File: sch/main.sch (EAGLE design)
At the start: 7 parts, among them U1 LTC3789EGNPBF

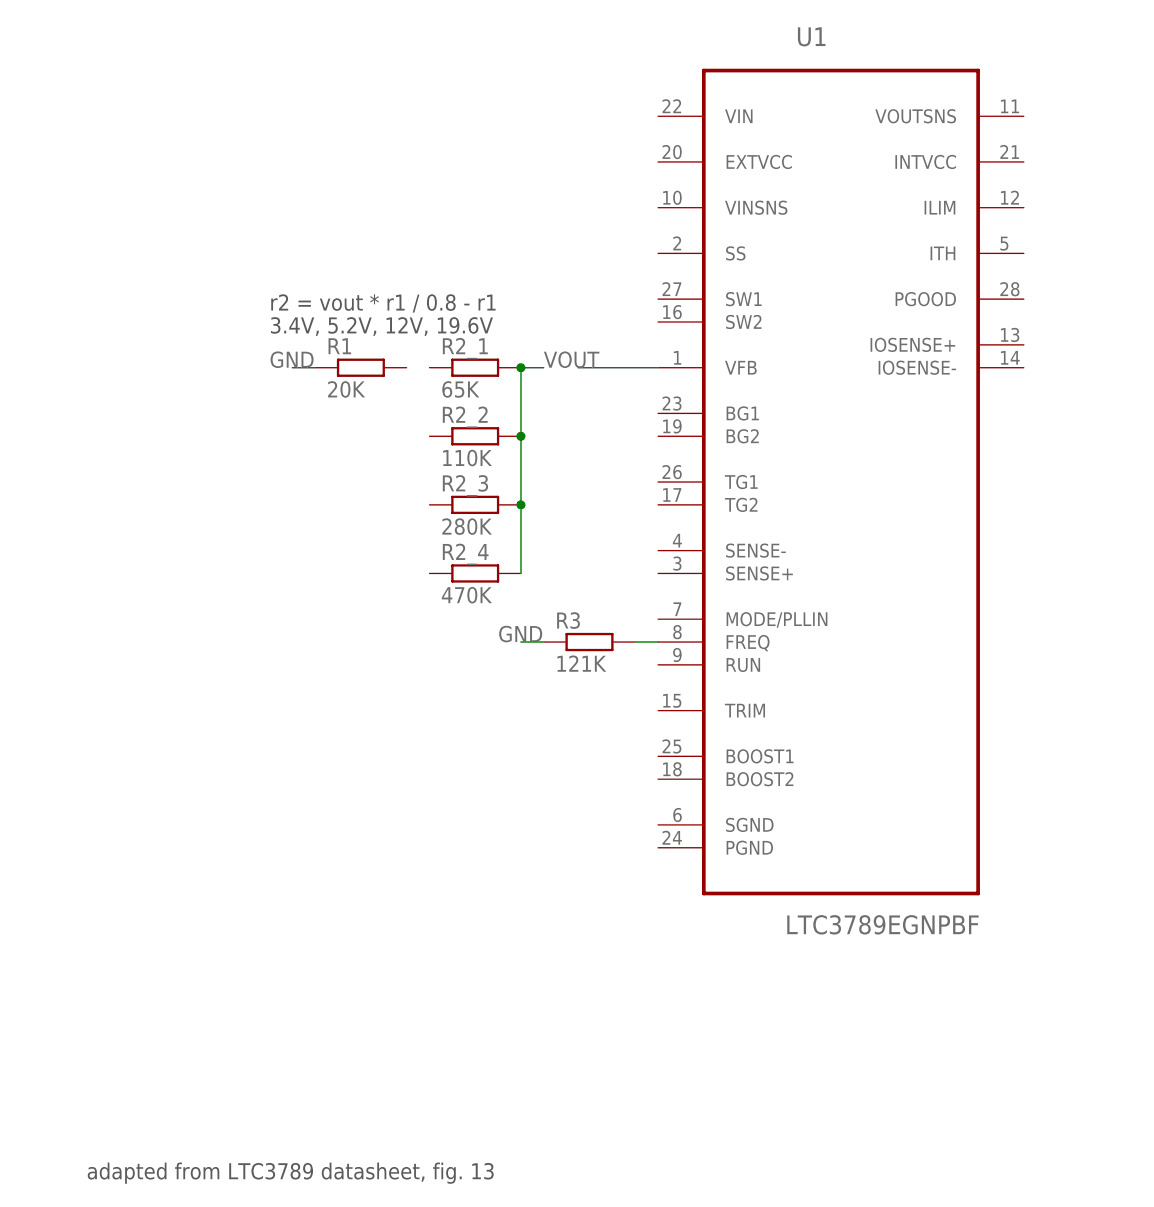
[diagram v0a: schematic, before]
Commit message: [ update ] sch
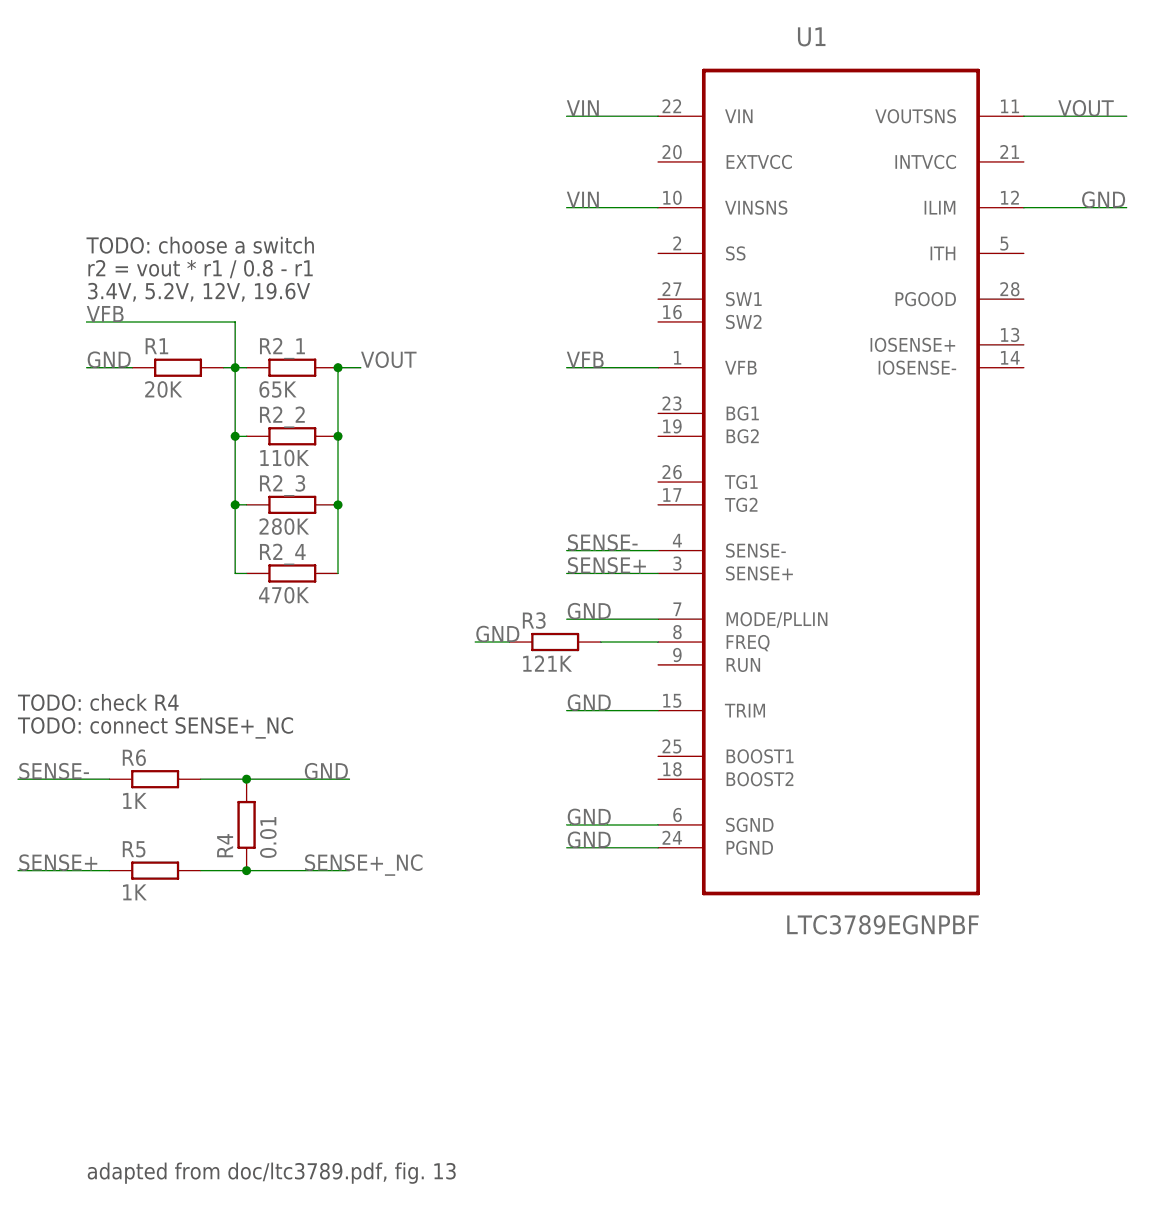
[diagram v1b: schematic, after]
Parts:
- added R4: 0.01, resistor:R-EU_R1206
- added R5, R6: 1K, resistor:R-EU_R1206
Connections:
- removed net N$3: U1.VFB
- new net SENSE+: R5.1, U1.SENSE+
- new net SENSE+_NC: R4.1, R5.2
- new net SENSE-: R6.1, U1.SENSE-
- new net VFB: R1.2, R2_1.1, R2_2.1, R2_3.1, R2_4.1, U1.VFB
- new net VIN: U1.VIN, U1.VINSNS
- net GND: now also R4.2, R6.2, U1.ILIM, U1.MODE/PLLIN, U1.PGND, U1.SGND, U1.TRIM
- net VOUT: now also U1.VOUTSNS
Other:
- note added: "TODO: check R4"
- note added: "TODO: choose a switch"
- note added: "TODO: connect SENSE+_NC"
- note added: "adapted from doc/ltc3789.pdf, fig. 13"
- note removed: "adapted from LTC3789 datasheet, fig. 13"
- moved on the sheet: R1, R2_1, R2_2, R2_3, R2_4, R3
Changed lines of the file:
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@@
 <part name="R2_3" library="resistor" deviceset="R-EU_" device="R1206" value="280K"/>
 <part name="R2_4" library="resistor" deviceset="R-EU_" device="R1206" value="470K"/>
+<part name="R4" library="resistor" deviceset="R-EU_" device="R1206" value="0.01"/>
+<part name="R6" library="resistor" deviceset="R-EU_" device="R1206" value="1K"/>
+<part name="R5" library="resistor" deviceset="R-EU_" device="R1206" value="1K"/>
 </parts>
 <sheets>
 <sheet>
 <plain>
-<text x="0" y="0" size="1.778" layer="97">adapted from LTC3789 datasheet, fig. 13</text>
-<text x="20.32" y="96.52" size="1.778" layer="97">r2 = vout * r1 / 0.8 - r1</text>
-<text x="20.32" y="93.98" size="1.778" layer="97">3.4V, 5.2V, 12V, 19.6V</text>
+<text x="0" y="0" size="1.778" layer="97">adapted from doc/ltc3789.pdf, fig. 13</text>
+<text x="0" y="100.33" size="1.778" layer="97">r2 = vout * r1 / 0.8 - r1</text>
+<text x="0" y="97.79" size="1.778" layer="97">3.4V, 5.2V, 12V, 19.6V</text>
+<text x="-7.62" y="52.07" size="1.778" layer="97">TODO: check R4</text>
+<text x="0" y="102.87" size="1.778" layer="97">TODO: choose a switch</text>
+<text x="-7.62" y="49.53" size="1.778" layer="97">TODO: connect SENSE+_NC</text>
 </plain>
 <instances>
 <instance part="U1" gate="A" x="83.82" y="80.01"/>
-<instance part="R3" gate="G$1" x="55.88" y="59.69"/>
-<instance part="R2_1" gate="G$1" x="43.18" y="90.17"/>
-<instance part="R1" gate="G$1" x="30.48" y="90.17"/>
-<instance part="R2_2" gate="G$1" x="43.18" y="82.55"/>
-<instance part="R2_3" gate="G$1" x="43.18" y="74.93"/>
-<instance part="R2_4" gate="G$1" x="43.18" y="67.31"/>
+<instance part="R3" gate="G$1" x="52.07" y="59.69"/>
+<instance part="R2_1" gate="G$1" x="22.86" y="90.17"/>
+<instance part="R1" gate="G$1" x="10.16" y="90.17"/>
+<instance part="R2_2" gate="G$1" x="22.86" y="82.55"/>
+<instance part="R2_3" gate="G$1" x="22.86" y="74.93"/>
+<instance part="R2_4" gate="G$1" x="22.86" y="67.31"/>
+<instance part="R4" gate="G$1" x="17.78" y="39.37" rot="R90"/>
+<instance part="R6" gate="G$1" x="7.62" y="44.45"/>
+<instance part="R5" gate="G$1" x="7.62" y="34.29"/>
 </instances>
 <busses>
@@
 <pinref part="R3" gate="G$1" pin="2"/>
 <pinref part="U1" gate="A" pin="FREQ"/>
-<wire x1="60.96" y1="59.69" x2="63.5" y2="59.69" width="0.1524" layer="91"/>
+<wire x1="57.15" y1="59.69" x2="63.5" y2="59.69" width="0.1524" layer="91"/>
 </segment>
 </net>
@@
 <segment>
 <pinref part="R3" gate="G$1" pin="1"/>
-<wire x1="50.8" y1="59.69" x2="48.26" y2="59.69" width="0.1524" layer="91"/>
-<label x="45.72" y="59.69" size="1.778" layer="95"/>
+<wire x1="46.99" y1="59.69" x2="43.18" y2="59.69" width="0.1524" layer="91"/>
+<label x="43.18" y="59.69" size="1.778" layer="95"/>
 </segment>
 <segment>
 <pinref part="R1" gate="G$1" pin="1"/>
-<wire x1="25.4" y1="90.17" x2="22.86" y2="90.17" width="0.1524" layer="91"/>
-<label x="20.32" y="90.17" size="1.778" layer="95"/>
+<wire x1="5.08" y1="90.17" x2="0" y2="90.17" width="0.1524" layer="91"/>
+<label x="0" y="90.17" size="1.778" layer="95"/>
+</segment>
+<segment>
+<pinref part="U1" gate="A" pin="SGND"/>
+<wire x1="63.5" y1="39.37" x2="53.34" y2="39.37" width="0.1524" layer="91"/>
+<label x="53.34" y="39.37" size="1.778" layer="95"/>
+</segment>
+<segment>
+<pinref part="U1" gate="A" pin="PGND"/>
+<wire x1="63.5" y1="36.83" x2="53.34" y2="36.83" width="0.1524" layer="91"/>
+<label x="53.34" y="36.83" size="1.778" layer="95"/>
+</segment>
+<segment>
+<pinref part="R4" gate="G$1" pin="2"/>
+<pinref part="R6" gate="G$1" pin="2"/>
+<wire x1="12.7" y1="44.45" x2="17.78" y2="44.45" width="0.1524" layer="91"/>
+<wire x1="17.78" y1="44.45" x2="29.21" y2="44.45" width="0.1524" layer="91"/>
+<junction x="17.78" y="44.45"/>
+<label x="24.13" y="44.45" size="1.778" layer="95"/>
+</segment>
+<segment>
+<pinref part="U1" gate="A" pin="ILIM"/>
+<wire x1="104.14" y1="107.95" x2="115.57" y2="107.95" width="0.1524" layer="91"/>
+<label x="110.49" y="107.95" size="1.778" layer="95"/>
+</segment>
+<segment>
+<pinref part="U1" gate="A" pin="MODE/PLLIN"/>
+<wire x1="63.5" y1="62.23" x2="53.34" y2="62.23" width="0.1524" layer="91"/>
+<label x="53.34" y="62.23" size="1.778" layer="95"/>
+</segment>
+<segment>
+<pinref part="U1" gate="A" pin="TRIM"/>
+<wire x1="63.5" y1="52.07" x2="53.34" y2="52.07" width="0.1524" layer="91"/>
+<label x="53.34" y="52.07" size="1.778" layer="95"/>
 </segment>
 </net>
@@
 <segment>
 <pinref part="R2_1" gate="G$1" pin="2"/>
-<wire x1="48.26" y1="90.17" x2="50.8" y2="90.17" width="0.1524" layer="91"/>
-<label x="50.8" y="90.17" size="1.778" layer="95"/>
+<wire x1="27.94" y1="90.17" x2="30.48" y2="90.17" width="0.1524" layer="91"/>
+<label x="30.48" y="90.17" size="1.778" layer="95"/>
 <pinref part="R2_2" gate="G$1" pin="2"/>
-<wire x1="48.26" y1="90.17" x2="48.26" y2="82.55" width="0.1524" layer="91"/>
-<junction x="48.26" y="90.17"/>
+<wire x1="27.94" y1="90.17" x2="27.94" y2="82.55" width="0.1524" layer="91"/>
+<junction x="27.94" y="90.17"/>
 <pinref part="R2_3" gate="G$1" pin="2"/>
-<wire x1="48.26" y1="82.55" x2="48.26" y2="74.93" width="0.1524" layer="91"/>
-<junction x="48.26" y="82.55"/>
+<wire x1="27.94" y1="82.55" x2="27.94" y2="74.93" width="0.1524" layer="91"/>
+<junction x="27.94" y="82.55"/>
 <pinref part="R2_4" gate="G$1" pin="2"/>
-<wire x1="48.26" y1="74.93" x2="48.26" y2="67.31" width="0.1524" layer="91"/>
-<junction x="48.26" y="74.93"/>
+<wire x1="27.94" y1="74.93" x2="27.94" y2="67.31" width="0.1524" layer="91"/>
+<junction x="27.94" y="74.93"/>
+</segment>
+<segment>
+<pinref part="U1" gate="A" pin="VOUTSNS"/>
+<wire x1="104.14" y1="118.11" x2="115.57" y2="118.11" width="0.1524" layer="91"/>
+<label x="107.95" y="118.11" size="1.778" layer="95"/>
 </segment>
 </net>
-<net name="N$3" class="0">
+<net name="VIN" class="0">
+<segment>
+<pinref part="U1" gate="A" pin="VIN"/>
+<wire x1="63.5" y1="118.11" x2="53.34" y2="118.11" width="0.1524" layer="91"/>
+<label x="53.34" y="118.11" size="1.778" layer="95"/>
+</segment>
+<segment>
+<pinref part="U1" gate="A" pin="VINSNS"/>
+<wire x1="63.5" y1="107.95" x2="53.34" y2="107.95" width="0.1524" layer="91"/>
+<label x="53.34" y="107.95" size="1.778" layer="95"/>
+</segment>
+</net>
+<net name="SENSE-" class="0">
+<segment>
+<pinref part="U1" gate="A" pin="SENSE-"/>
+<wire x1="63.5" y1="69.85" x2="53.34" y2="69.85" width="0.1524" layer="91"/>
+<label x="53.34" y="69.85" size="1.778" layer="95"/>
+</segment>
+<segment>
+<pinref part="R6" gate="G$1" pin="1"/>
+<wire x1="2.54" y1="44.45" x2="-7.62" y2="44.45" width="0.1524" layer="91"/>
+<label x="-7.62" y="44.45" size="1.778" layer="95"/>
+</segment>
+</net>
+<net name="SENSE+" class="0">
+<segment>
+<pinref part="U1" gate="A" pin="SENSE+"/>
+<wire x1="63.5" y1="67.31" x2="53.34" y2="67.31" width="0.1524" layer="91"/>
+<label x="53.34" y="67.31" size="1.778" layer="95"/>
+</segment>
+<segment>
+<pinref part="R5" gate="G$1" pin="1"/>
+<wire x1="2.54" y1="34.29" x2="-7.62" y2="34.29" width="0.1524" layer="91"/>
+<label x="-7.62" y="34.29" size="1.778" layer="95"/>
+</segment>
+</net>
+<net name="VFB" class="0">
+<segment>
+<pinref part="R2_1" gate="G$1" pin="1"/>
+<pinref part="R1" gate="G$1" pin="2"/>
+<wire x1="17.78" y1="90.17" x2="16.51" y2="90.17" width="0.1524" layer="91"/>
+<wire x1="16.51" y1="90.17" x2="15.24" y2="90.17" width="0.1524" layer="91"/>
+<wire x1="16.51" y1="90.17" x2="16.51" y2="95.25" width="0.1524" layer="91"/>
+<junction x="16.51" y="90.17"/>
+<wire x1="16.51" y1="95.25" x2="0" y2="95.25" width="0.1524" layer="91"/>
+<label x="0" y="95.25" size="1.778" layer="95"/>
+<wire x1="16.51" y1="90.17" x2="16.51" y2="82.55" width="0.1524" layer="91"/>
+<pinref part="R2_4" gate="G$1" pin="1"/>
+<wire x1="16.51" y1="82.55" x2="16.51" y2="74.93" width="0.1524" layer="91"/>
+<wire x1="16.51" y1="74.93" x2="16.51" y2="67.31" width="0.1524" layer="91"/>
+<wire x1="16.51" y1="67.31" x2="17.78" y2="67.31" width="0.1524" layer="91"/>
+<pinref part="R2_3" gate="G$1" pin="1"/>
+<wire x1="17.78" y1="74.93" x2="16.51" y2="74.93" width="0.1524" layer="91"/>
+<junction x="16.51" y="74.93"/>
+<pinref part="R2_2" gate="G$1" pin="1"/>
+<wire x1="16.51" y1="82.55" x2="17.78" y2="82.55" width="0.1524" layer="91"/>
+<junction x="16.51" y="82.55"/>
+</segment>
 <segment>
 <pinref part="U1" gate="A" pin="VFB"/>
-<wire x1="63.5" y1="90.17" x2="54.61" y2="90.17" width="0.1524" layer="91"/>
+<wire x1="63.5" y1="90.17" x2="53.34" y2="90.17" width="0.1524" layer="91"/>
+<label x="53.34" y="90.17" size="1.778" layer="95"/>
 </segment>
 </net>
+<net name="SENSE+_NC" class="0">
+<segment>
+<pinref part="R4" gate="G$1" pin="1"/>
+<wire x1="17.78" y1="34.29" x2="12.7" y2="34.29" width="0.1524" layer="91"/>
+<pinref part="R5" gate="G$1" pin="2"/>
+<wire x1="17.78" y1="34.29" x2="29.21" y2="34.29" width="0.1524" layer="91"/>
+<junction x="17.78" y="34.29"/>
+<label x="24.13" y="34.29" size="1.778" layer="95"/>
+</segment>
+</net>
